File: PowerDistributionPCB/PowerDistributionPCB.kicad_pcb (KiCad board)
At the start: 4 copper layers, 92.3 x 122.5 mm, 87 parts, among them K1 RT314F05(gen), K2 RT314F05(gen), K3 RT314F05(gen), K4 RT314F05(gen), Q1 AOD4185, Q10 MMBT2222A, Q11 MMBT2222A, Q12 MMBT2222A, Q2 MMBT2222A, Q6 MMBT2222A, Q7 MMBT2222A, Q8 MMBT2222A, Q9 MMBT2222A, U1 AP63203WU

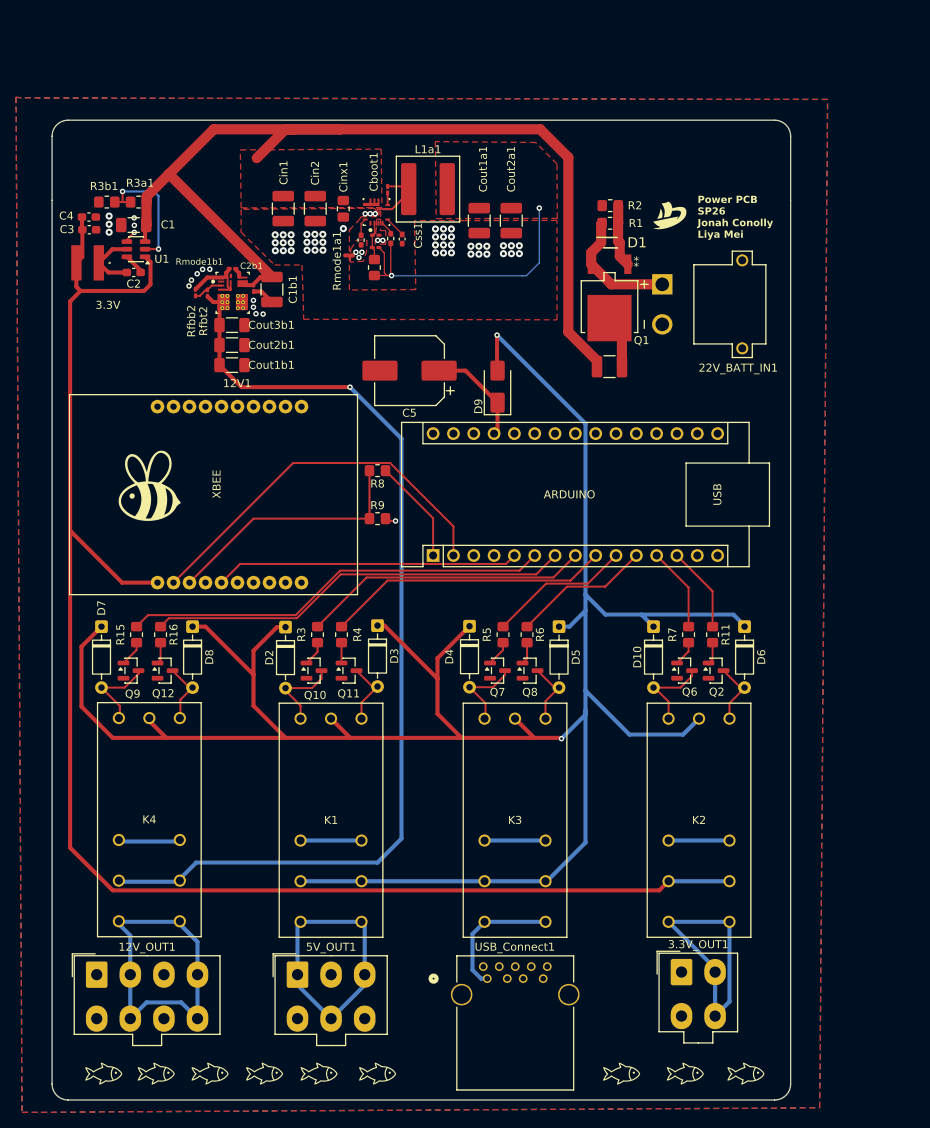
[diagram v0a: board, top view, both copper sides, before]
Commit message: finished final updates
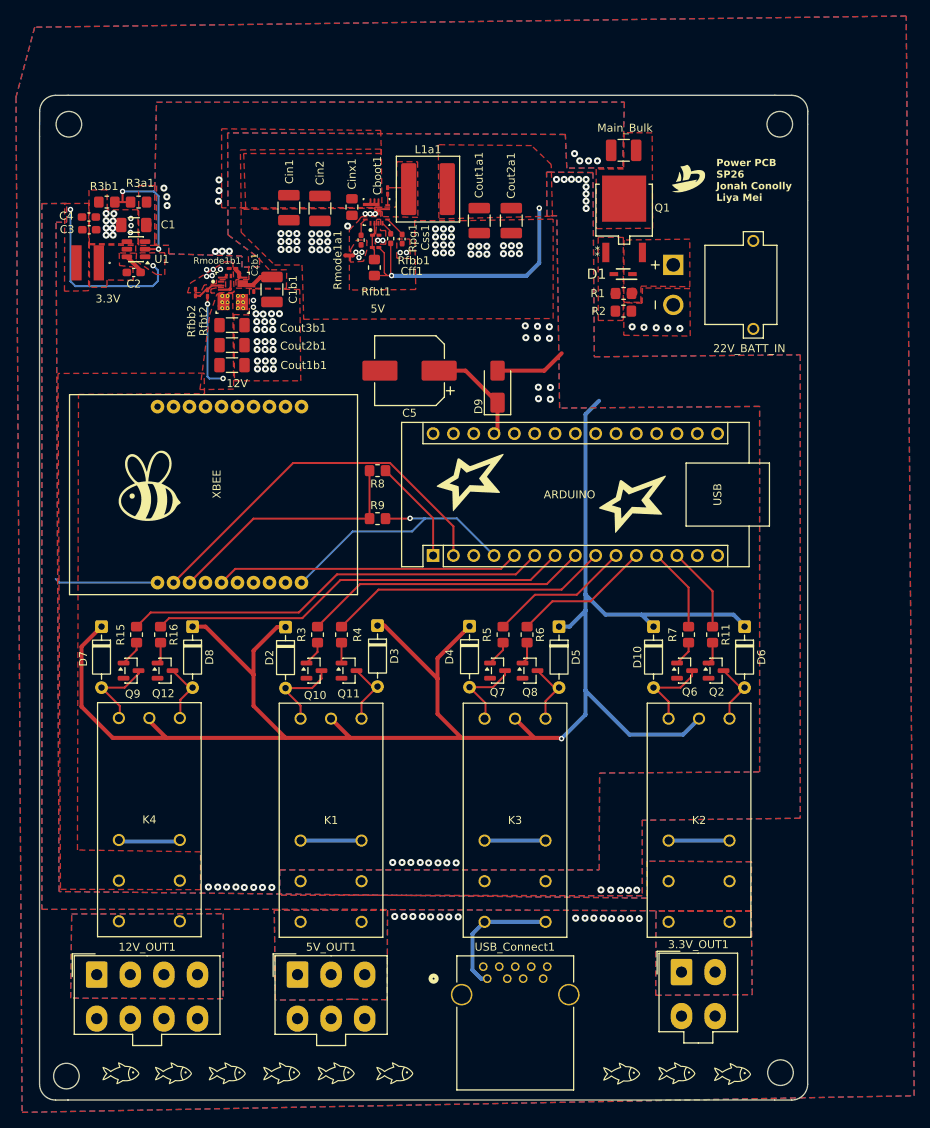
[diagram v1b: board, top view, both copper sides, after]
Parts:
- added G***: LOGO, LOGO, F.Cu at (126.5, 84.1)
- added G***: LOGO, LOGO, F.Cu at (106.2, 81.3)
- added H1: MountingHole, MountingHole:MountingHole_3.2mm_M3, F.Cu at (55.6, 36.9)
- added H2: MountingHole, MountingHole:MountingHole_3.2mm_M3, F.Cu at (144.5, 36.9)
- added H3: MountingHole, MountingHole:MountingHole_3.2mm_M3, F.Cu at (55.3, 155.9)
- added H4: MountingHole, MountingHole:MountingHole_3.2mm_M3, F.Cu at (144.6, 155.4)
- moved Main_Bulk 27.1 mm to (125.0, 40.1)
- moved R2 13.3 mm to (124.9, 60.3), turned to 180 degrees
- moved Q1 12.2 mm to (125.0, 47.6), turned to 0 degrees
- moved R1 8.93 mm to (124.9, 58.0), turned to 180 degrees
- moved G*** 5.17 mm to (133.1, 43.7)
- moved D1 4.24 mm to (124.9, 55.6), turned to 180 degrees
- moved 22V_BATT_IN 2.80 mm to (141.2, 57.0)
- moved G*** 2.15 mm to (68.7, 155.5)
- moved G*** 2.15 mm to (89.0, 155.5)
- moved G*** 2.15 mm to (82.2, 155.5)
- moved G*** 2.15 mm to (62.1, 155.5)
- moved G*** 2.15 mm to (75.4, 155.5)
- moved G*** 2.15 mm to (96.3, 155.5)
- moved G*** 1.67 mm to (138.6, 155.6)
- moved Cinx1 1.10 mm to (91.0, 47.2)
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- renumbered 12V1 to 12V, 22V_BATT_IN1 to 22V_BATT_IN, Main_Bulk(electrolytic)1 to Main_Bulk
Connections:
- 12V_OUT1 pad 1: GND -> 12VRelayOut
- 12V_OUT1 pad 3: GND -> 12VRelayOut
- 12V_OUT1 pad 6: 12VRelayOut -> GND
- 12V_OUT1 pad 8: 12VRelayOut -> GND
- 3.3V_OUT1 pad 1: GND -> 3.3VRelayOut
- 3.3V_OUT1 pad 4: 3.3VRelayOut -> GND
- 5V_OUT1 pad 2: GND -> 5VRelayOut
- 5V_OUT1 pad 5: 5VRelayOut -> GND
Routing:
- net 3.3VBuck: track 191.5 -> 35.6 mm, vias 0 -> 2
- net Sys_Vin: track 124.8 -> 3.86 mm, vias 0 -> 13
- net 12VBuck: track 125.0 -> 12.9 mm, vias 1 -> 2
- net 5VBuck: track 334.1 -> 272.5 mm, vias 4 -> 17
- net 12VRelayOut: track 43.7 -> 0.00 mm
- net 3.3VRelayOut: track 34.3 -> 0.46 mm
- net 5VRelayOut: track 35.6 -> 3.70 mm
- net Batt_Vin: track 15.6 -> 0.16 mm
- net Net-(U1-SW): track 8.22 -> 0.00 mm
- net GND: track 29.2 -> 37.3 mm, vias 53 -> 134
- net Net-(D1-A): track 7.84 -> 0.03 mm
- net Net-(Q1-D): track 6.84 -> 3.08 mm
- net Net-(5V1-SW): track 7.24 -> 3.62 mm
- net VNRelayOut: track 17.1 -> 16.6 mm
- net Net-(D8-A): track 8.04 -> 7.53 mm
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- added copper zone on F.Cu, net 12VBuck
- added copper zone on In2.Cu, net 12VBuck
- added copper zone on B.Cu, net 12VRelayOut
- added copper zone on F.Cu, net 12VRelayOut
- added copper zone on In2.Cu, net 12VRelayOut
- added copper zone on B.Cu, net 3.3VBuck
- added copper zone on F.Cu, net 3.3VBuck
- added copper zone on In2.Cu, net 3.3VBuck
- added copper zone on B.Cu, net 3.3VRelayOut
- added copper zone on F.Cu, net 3.3VRelayOut
- added copper zone on In2.Cu, net 3.3VRelayOut
- added copper zone on B.Cu, net 5VBuck
- added copper zone on In2.Cu, net 5VBuck
- added copper zone on B.Cu, net 5VRelayOut
- added copper zone on F.Cu, net 5VRelayOut
- added copper zone on In2.Cu, net 5VRelayOut
- added copper zone on F.Cu, net Batt_Vin
- added copper zone on F.Cu, net Net-(5V1-SW)
- added copper zone on F.Cu, net Net-(D1-A)
- added copper zone on F.Cu, net Net-(Q1-D)
- added copper zone on F.Cu, net Net-(U1-SW)
- added copper zone on B.Cu, net Sys_Vin
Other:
- board size 92.3 x 122.5 mm -> 96 x 125.6 mm
- board text added: "5V"
